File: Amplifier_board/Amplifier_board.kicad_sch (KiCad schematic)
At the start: 15 parts, among them J1 Screw Terminal, J2 Screw Terminal, J3 Screw Terminal, J4 Screw Terminal, J5 Screw Terminal, J6 Screw Terminal, J7 Conn_02x04_Odd_Even

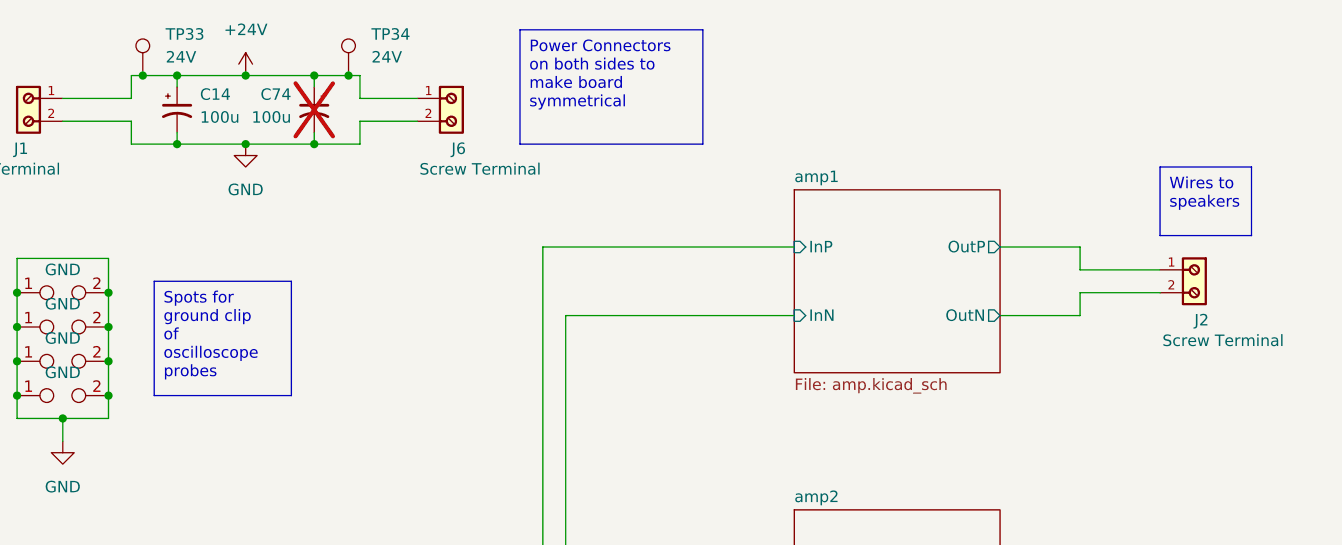
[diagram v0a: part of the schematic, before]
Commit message: generated gerber files
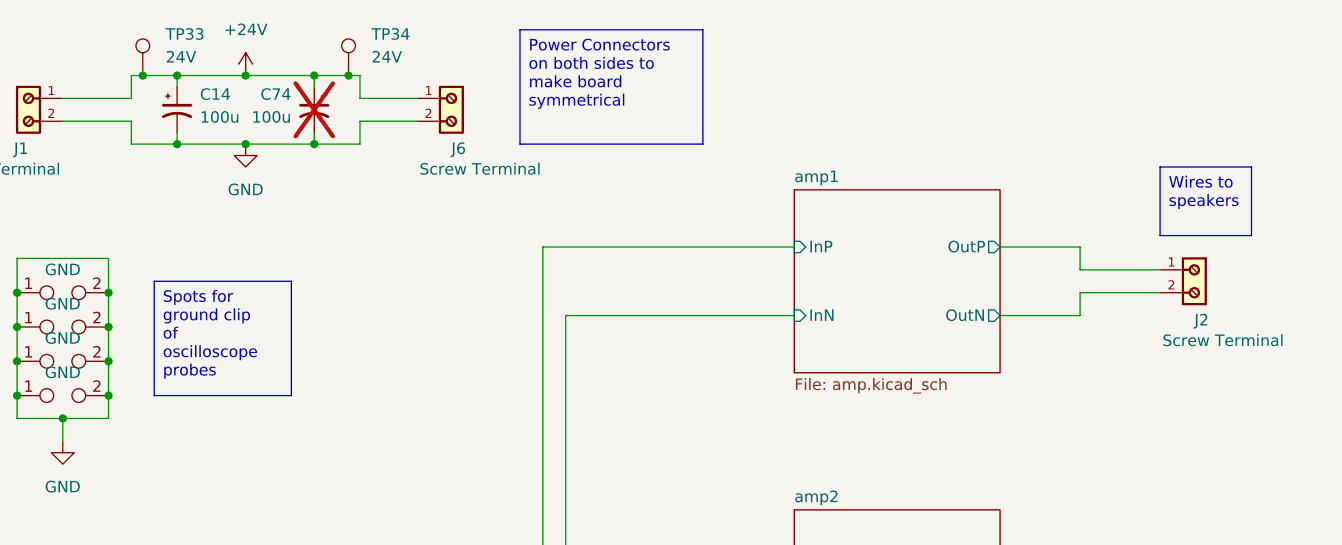
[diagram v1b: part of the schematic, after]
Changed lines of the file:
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@@
 (kicad_sch
-	(version 20231120)
+	(version 20250114)
 	(generator "eeschema")
-	(generator_version "8.0")
+	(generator_version "9.0")
 	(paper "A4")
+	(text_box "Wires to speakers\n"
+		(exclude_from_sim no)
+		(at 152.4 33.02 0)
+		(size 10.16 7.62)
+		(margins 0.9525 0.9525 0.9525 0.9525)
+		(stroke
+			(width 0)
+			(type default)
+		)
+		(fill
+			(type none)
+		)
+		(effects
+			(font
+				(size 1.27 1.27)
+			)
+			(justify left top)
+		)
+	)
+	(text_box "Spots for ground clip of oscilloscope probes"
+		(exclude_from_sim no)
+		(at 40.64 45.72 0)
+		(size 15.24 12.7)
+		(margins 0.9525 0.9525 0.9525 0.9525)
+		(stroke
+			(width 0)
+			(type default)
+		)
+		(fill
+			(type none)
+		)
+		(effects
+			(font
+				(size 1.27 1.27)
+			)
+			(justify left top)
+		)
+	)
+	(text_box "Power Connectors on both sides to make board symmetrical\n"
+		(exclude_from_sim no)
+		(at 81.28 17.78 0)
+		(size 20.32 12.7)
+		(margins 0.9525 0.9525 0.9525 0.9525)
+		(stroke
+			(width 0)
+			(type default)
+		)
+		(fill
+			(type none)
+		)
+		(effects
+			(font
+				(size 1.27 1.27)
+			)
+			(justify left top)
+		)
+	)
 	(junction
 		(at 35.56 46.99)
@@
 		)
 	)
-	(text_box "Wires to speakers\n"
-		(exclude_from_sim no)
-		(at 152.4 33.02 0)
-		(size 10.16 7.62)
-		(stroke
-			(width 0)
-			(type default)
-		)
-		(fill
-			(type none)
-		)
+	(label "In2N"
+		(at 67.31 96.52 0)
 		(effects
 			(font
 				(size 1.27 1.27)
 			)
-			(justify left top)
-		)
-	)
-	(text_box "Spots for ground clip of oscilloscope probes"
-		(exclude_from_sim no)
-		(at 40.64 45.72 0)
-		(size 15.24 12.7)
-		(stroke
-			(width 0)
-			(type default)
-		)
-		(fill
-			(type none)
-		)
+			(justify left bottom)
+		)
+	)
+	(label "In1N"
+		(at 52.07 93.98 0)
 		(effects
 			(font
 				(size 1.27 1.27)
 			)
-			(justify left top)
-		)
-	)
-	(text_box "Power Connectors on both sides to make board symmetrical\n"
-		(exclude_from_sim no)
-		(at 81.28 17.78 0)
-		(size 20.32 12.7)
-		(stroke
-			(width 0)
-			(type default)
-		)
-		(fill
-			(type none)
-		)
+			(justify left bottom)
+		)
+	)
+	(label "In4N"
+		(at 67.31 106.68 0)
 		(effects
 			(font
 				(size 1.27 1.27)
 			)
-			(justify left top)
-		)
-	)
-	(label "In2N"
-		(at 67.31 96.52 0)
-		(fields_autoplaced yes)
+			(justify left bottom)
+		)
+	)
+	(label "In1P"
+		(at 67.31 88.9 0)
 		(effects
 			(font
@@
 		)
 	)
-	(label "In1N"
-		(at 52.07 93.98 0)
-		(fields_autoplaced yes)
+	(label "In4N"
+		(at 52.07 101.6 0)
 		(effects
 			(font
@@
 		)
 	)
-	(label "In4N"
-		(at 67.31 106.68 0)
-		(fields_autoplaced yes)
+	(label "In4P"
+		(at 34.29 101.6 180)
 		(effects
 			(font
 				(size 1.27 1.27)
 			)
-			(justify left bottom)
-		)
-	)
-	(label "In1P"
-		(at 67.31 88.9 0)
-		(fields_autoplaced yes)
+			(justify right bottom)
+		)
+	)
+	(label "In4P"
+		(at 67.31 104.14 0)
 		(effects
 			(font
@@
 		)
 	)
-	(label "In4N"
-		(at 52.07 101.6 0)
-		(fields_autoplaced yes)
+	(label "In3N"
+		(at 67.31 101.6 0)
 		(effects
 			(font
@@
 		)
 	)
-	(label "In4P"
-		(at 34.29 101.6 180)
-		(fields_autoplaced yes)
+	(label "In2N"
+		(at 52.07 96.52 0)
 		(effects
 			(font
 				(size 1.27 1.27)
 			)
-			(justify right bottom)
-		)
-	)
-	(label "In4P"
-		(at 67.31 104.14 0)
-		(fields_autoplaced yes)
+			(justify left bottom)
+		)
+	)
+	(label "In1N"
+		(at 67.31 91.44 0)
 		(effects
 			(font
@@
 		)
 	)
-	(label "In3N"
-		(at 67.31 101.6 0)
-		(fields_autoplaced yes)
+	(label "In2P"
+		(at 34.29 96.52 180)
 		(effects
 			(font
 				(size 1.27 1.27)
 			)
-			(justify left bottom)
-		)
-	)
-	(label "In2N"
-		(at 52.07 96.52 0)
-		(fields_autoplaced yes)
+			(justify right bottom)
+		)
+	)
+	(label "In1P"
+		(at 34.29 93.98 180)
 		(effects
 			(font
 				(size 1.27 1.27)
 			)
-			(justify left bottom)
-		)
-	)
-	(label "In1N"
-		(at 67.31 91.44 0)
-		(fields_autoplaced yes)
+			(justify right bottom)
+		)
+	)
+	(label "In3N"
+		(at 52.07 99.06 0)
 		(effects
 			(font
@@
 	)
 	(label "In2P"
-		(at 34.29 96.52 180)
-		(fields_autoplaced yes)
+		(at 67.31 93.98 0)
 		(effects
 			(font
 				(size 1.27 1.27)
 			)
-			(justify right bottom)
-		)
-	)
-	(label "In1P"
-		(at 34.29 93.98 180)
-		(fields_autoplaced yes)
+			(justify left bottom)
+		)
+	)
+	(label "In3P"
+		(at 67.31 99.06 0)
 		(effects
 			(font
 				(size 1.27 1.27)
 			)
-			(justify right bottom)
-		)
-	)
-	(label "In3N"
-		(at 52.07 99.06 0)
-		(fields_autoplaced yes)
-		(effects
-			(font
-				(size 1.27 1.27)
-			)
-			(justify left bottom)
-		)
-	)
-	(label "In2P"
-		(at 67.31 93.98 0)
-		(fields_autoplaced yes)
-		(effects
-			(font
-				(size 1.27 1.27)
-			)
-			(justify left bottom)
-		)
-	)
-	(label "In3P"
-		(at 67.31 99.06 0)
-		(fields_autoplaced yes)
-		(effects
-			(font
-				(size 1.27 1.27)
-			)
 			(justify left bottom)
 		)
@@
 	(label "In3P"
 		(at 34.29 99.06 180)
-		(fields_autoplaced yes)
 		(effects
 			(font
@@
 		(at 111.76 139.7)
 		(size 22.86 20.32)
+		(exclude_from_sim no)
+		(in_bom yes)
+		(on_board yes)
+		(dnp no)
 		(fields_autoplaced yes)
 		(stroke
@@
 		(at 111.76 35.56)
 		(size 22.86 20.32)
+		(exclude_from_sim no)
+		(in_bom yes)
+		(on_board yes)
+		(dnp no)
 		(fields_autoplaced yes)
 		(stroke
@@
 		(at 111.76 104.14)
 		(size 22.86 20.32)
+		(exclude_from_sim no)
+		(in_bom yes)
+		(on_board yes)
+		(dnp no)
 		(fields_autoplaced yes)
 		(stroke
@@
 		(at 111.76 71.12)
 		(size 22.86 20.32)
+		(exclude_from_sim no)
+		(in_bom yes)
+		(on_board yes)
+		(dnp no)
 		(fields_autoplaced yes)
 		(stroke
@@
 		)
 	)
+	(embedded_fonts no)
 )
